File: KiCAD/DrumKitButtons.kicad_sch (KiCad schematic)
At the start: 6 parts, among them J1 Input, J2 Output

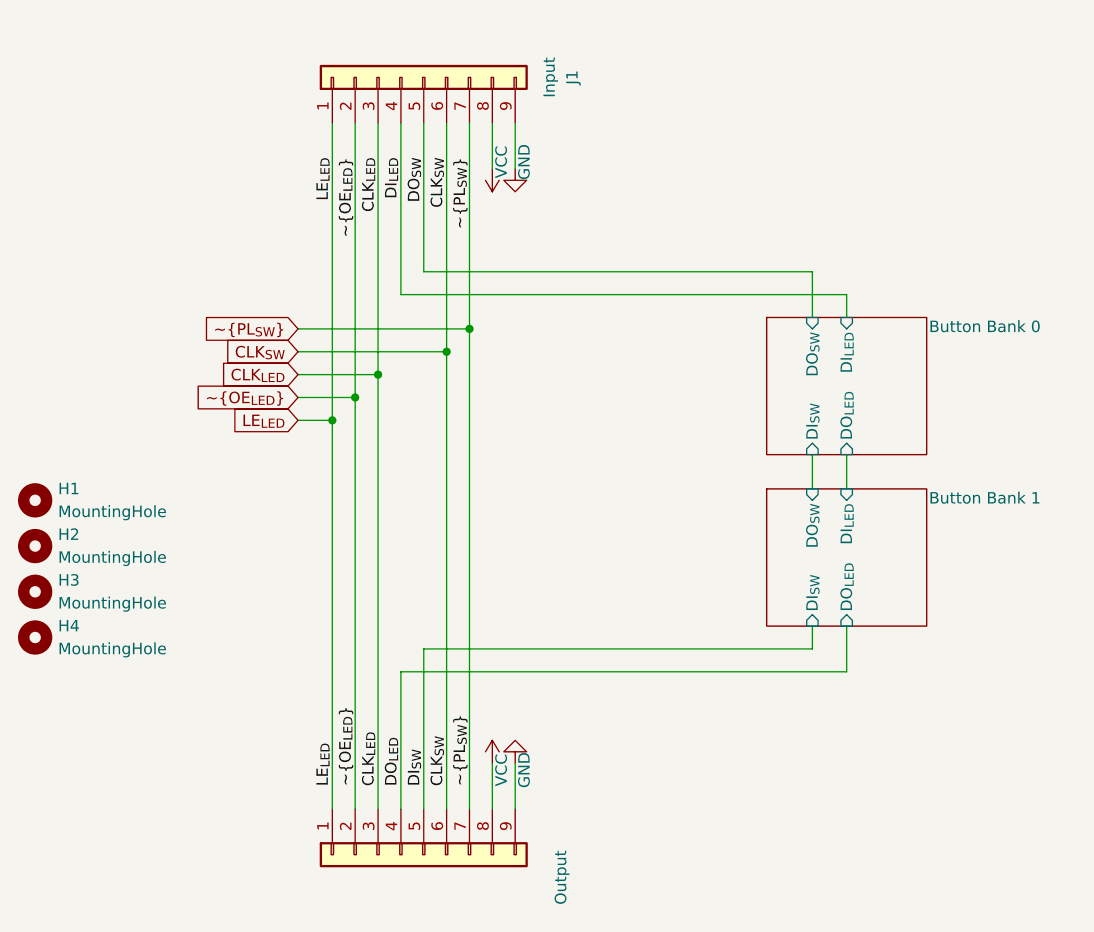
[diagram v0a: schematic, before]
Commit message: fix DRC errors
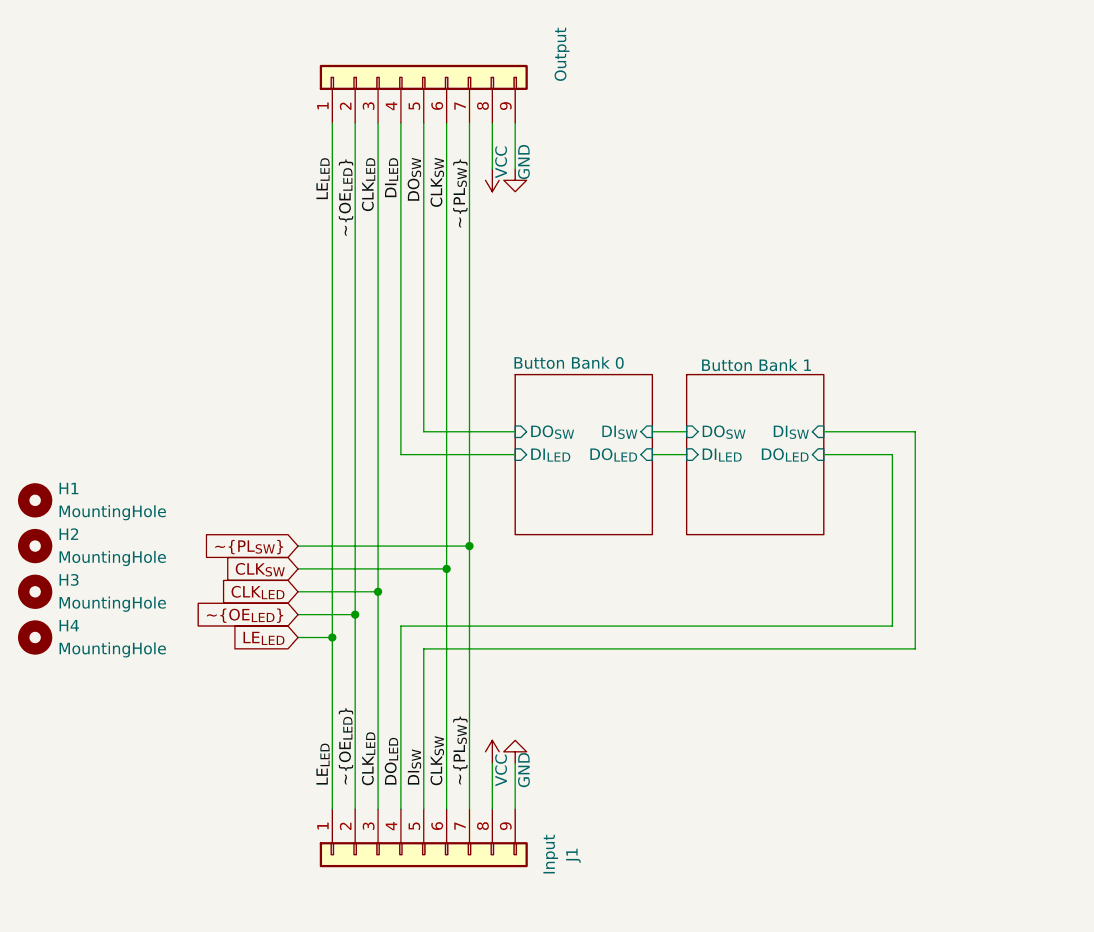
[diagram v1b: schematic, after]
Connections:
- net DI_{LED}: now also J2.4 (Pin_4); no longer J1.4 (Pin_4)
- net DI_{SW}: now also J1.5 (Pin_5); no longer J2.5 (Pin_5)
- net DO_{LED}: now also J1.4 (Pin_4); no longer J2.4 (Pin_4)
- net DO_{SW}: now also J2.5 (Pin_5); no longer J1.5 (Pin_5)
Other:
- moved on the sheet: J1
